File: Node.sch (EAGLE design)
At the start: 72 parts, among them J1 AVR_SPI_PRG_6NS, J2 M04X2, Q1 PMR280UN, Q2 PMR280UN, Q3 PMR280UN, SW1 KSS, U1 ATMEGA32U4, U2 BLUETOOTH-RN41", U4 L3GD20, U9 RCLAMP0502A, X1 USBSMD

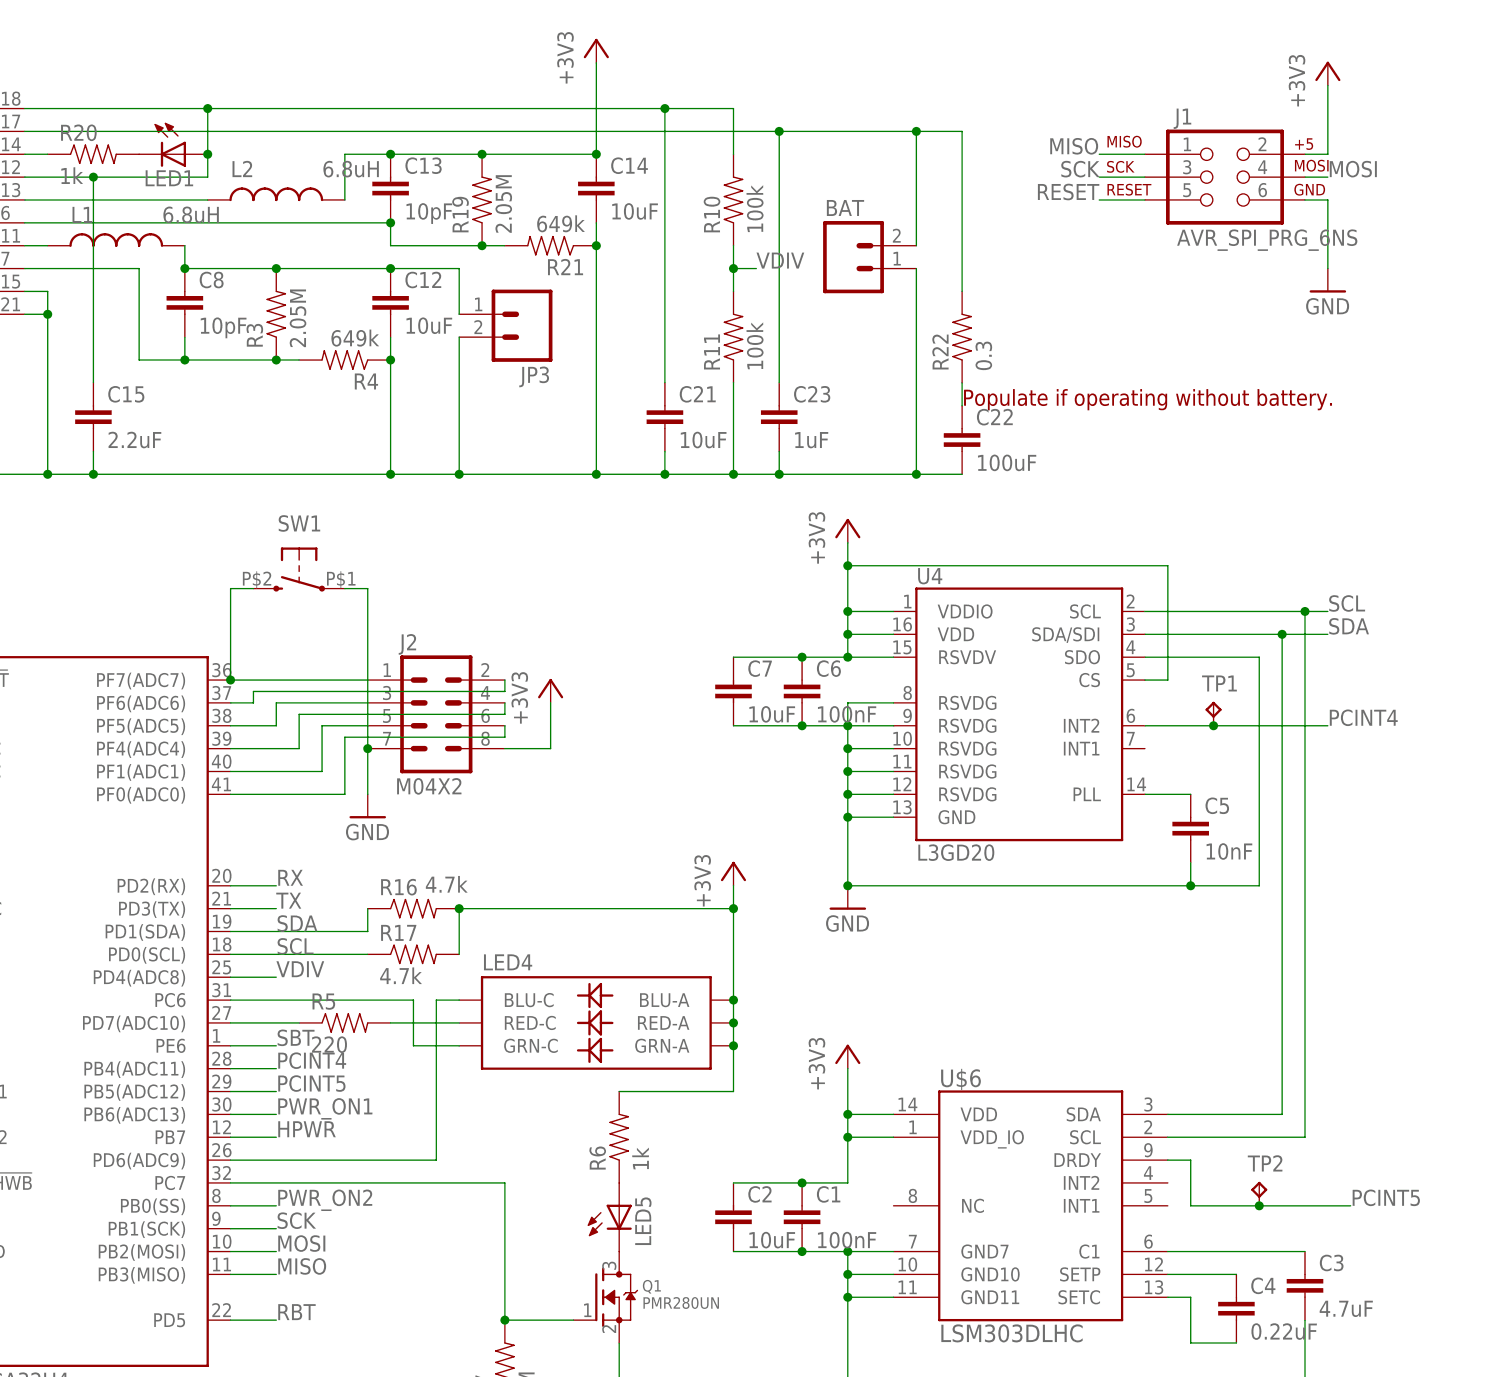
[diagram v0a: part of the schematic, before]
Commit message: it all sort of fits in the box
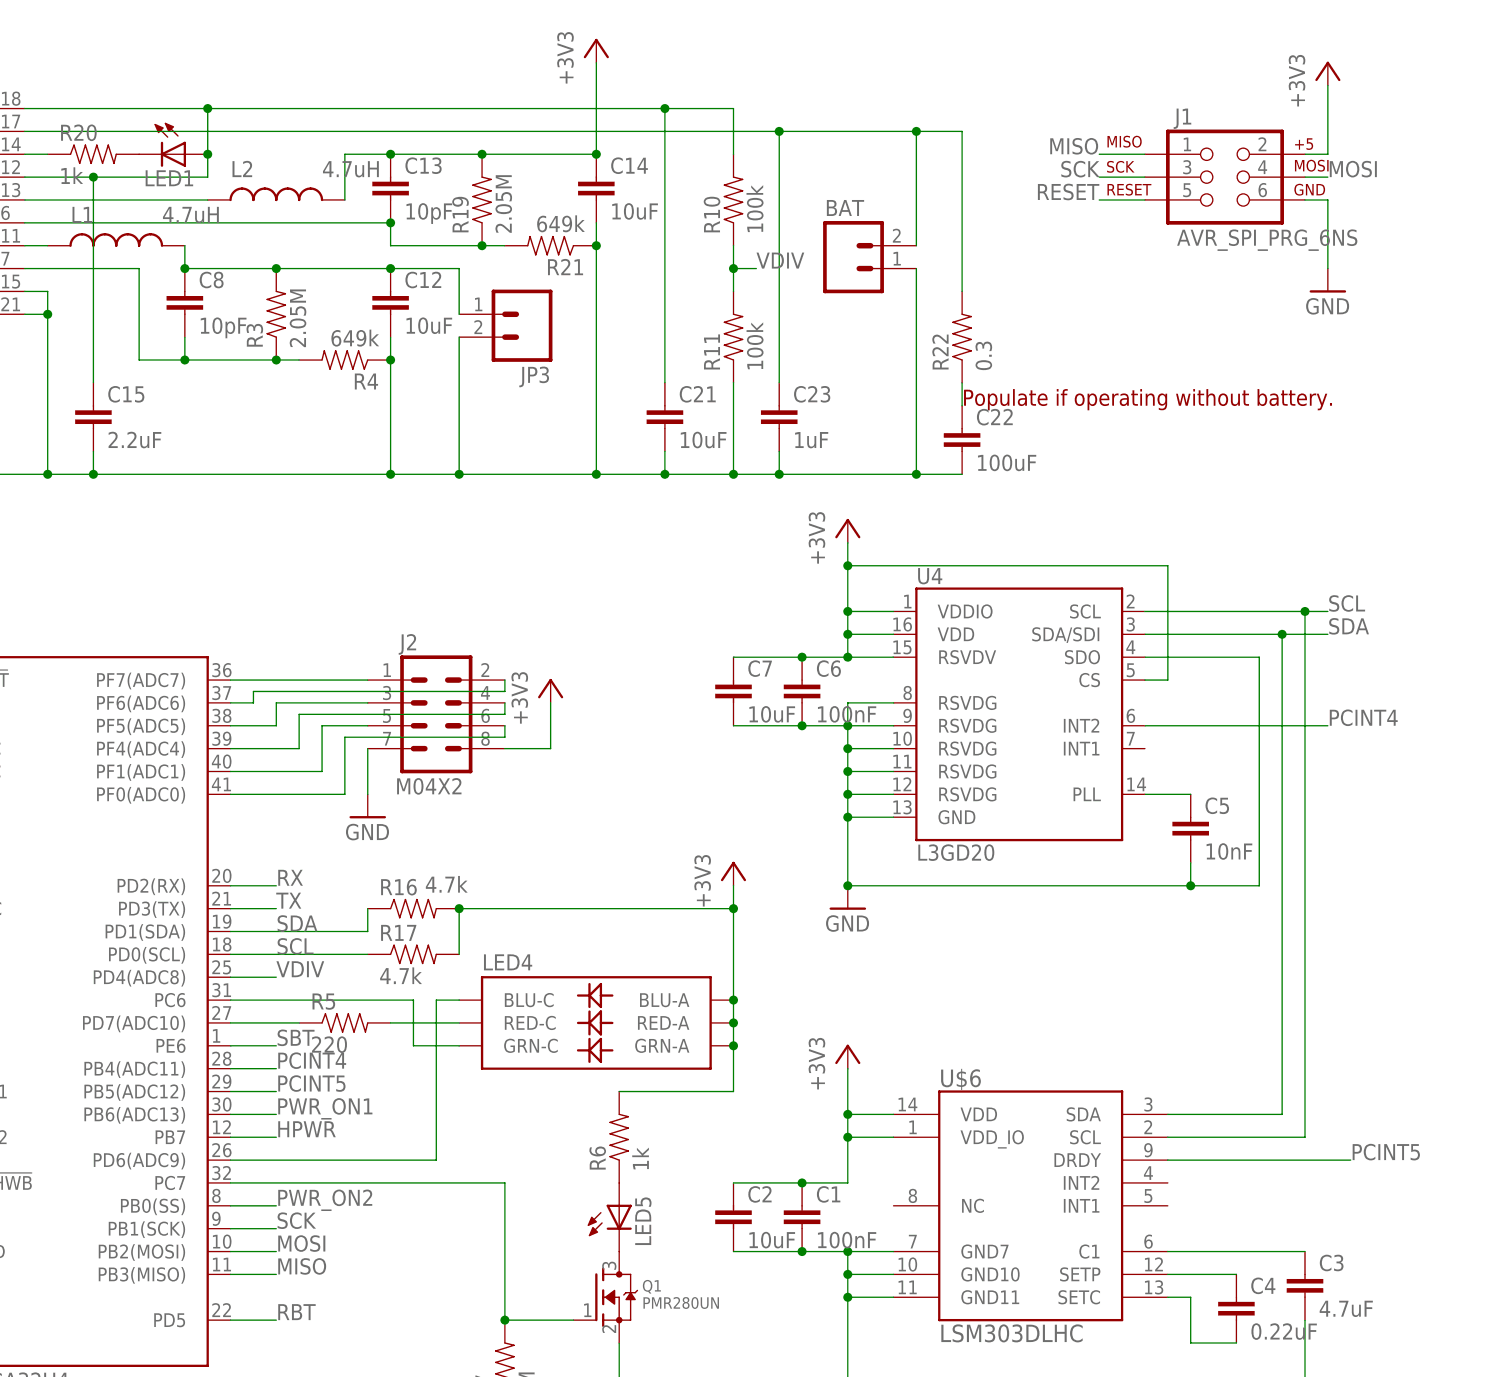
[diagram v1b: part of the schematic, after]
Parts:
- removed SW1: KSS, adjacent-reality:KSS
- removed TP1, TP2: TPTP06R, testpad:TPTP06R
- L1, L2: value 6.8uH -> 4.7uH; device adjacent-reality:INDUCTOR -> adjacent-reality:INDUCTORVLS2016
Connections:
- net GND: no longer SW1.1
- net N$28: no longer SW1.3
- net PCINT4: no longer TP1.TP
- net PCINT5: no longer TP2.TP
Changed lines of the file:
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@@
 <part name="R9" library="SparkFun" deviceset="RESISTOR" device="0402-RES" value="22"/>
 <part name="GND7" library="supply1" deviceset="GND" device=""/>
-<part name="SW1" library="adjacent-reality" deviceset="KSS" device=""/>
 <part name="HWB" library="adjacent-reality" deviceset="KSS" device=""/>
 <part name="C16" library="SparkFun" deviceset="CAP" device="0402-CAP" value="100nF"/>
@@
 <part name="R18" library="SparkFun" deviceset="RESISTOR" device="0402-RES" value="10k"/>
 <part name="U9" library="adjacent-reality" deviceset="RCLAMP0502A" device=""/>
-<part name="TP1" library="testpad" deviceset="TP" device="TP06R"/>
-<part name="TP2" library="testpad" deviceset="TP" device="TP06R"/>
 <part name="GND9" library="supply1" deviceset="GND" device=""/>
 <part name="LED1" library="SparkFun" deviceset="LED" device="0603"/>
@@
 <part name="C23" library="SparkFun" deviceset="CAP" device="0402-CAP" value="1uF"/>
 <part name="U$6" library="adjacent-reality" deviceset="LSM303DLHC" device=""/>
-<part name="L1" library="adjacent-reality" deviceset="INDUCTOR" device="" value="6.8uH"/>
-<part name="L2" library="adjacent-reality" deviceset="INDUCTOR" device="" value="6.8uH"/>
+<part name="L1" library="adjacent-reality" deviceset="INDUCTOR" device="VLS2016" value="4.7uH"/>
+<part name="L2" library="adjacent-reality" deviceset="INDUCTOR" device="VLS2016" value="4.7uH"/>
 <part name="JP1" library="SparkFun-Connectors" deviceset="M02" device="PTH"/>
 </parts>
@@
 <instance part="R9" gate="G$1" x="73.66" y="96.52"/>
 <instance part="GND7" gate="1" x="33.02" y="91.44"/>
-<instance part="SW1" gate="G$1" x="147.32" y="144.78" rot="MR0"/>
 <instance part="HWB" gate="G$1" x="48.26" y="134.62" smashed="yes" rot="MR0">
 <attribute name="NAME" x="50.8" y="140.97" size="1.778" layer="95" rot="MR0"/>
@@
 <instance part="R18" gate="G$1" x="55.88" y="139.7" rot="R90"/>
 <instance part="U9" gate="G$1" x="50.8" y="99.06"/>
-<instance part="TP1" gate="G$1" x="248.92" y="132.08"/>
-<instance part="TP2" gate="G$1" x="254" y="78.74"/>
 <instance part="GND9" gate="1" x="154.94" y="119.38"/>
 <instance part="LED1" gate="G$1" x="134.62" y="193.04" rot="R270"/>
@@
 <pinref part="J2" gate="G$1" pin="7"/>
 <wire x1="154.94" y1="121.92" x2="154.94" y2="127" width="0.1524" layer="91"/>
-<wire x1="154.94" y1="144.78" x2="154.94" y2="127" width="0.1524" layer="91"/>
-<junction x="154.94" y="127"/>
-<pinref part="SW1" gate="G$1" pin="1"/>
-<wire x1="154.94" y1="144.78" x2="152.4" y2="144.78" width="0.1524" layer="91"/>
 </segment>
 </net>
@@
 <segment>
 <pinref part="U4" gate="G$1" pin="INT2"/>
-<wire x1="241.3" y1="129.54" x2="248.92" y2="129.54" width="0.1524" layer="91"/>
 <label x="261.62" y="129.54" size="1.778" layer="95"/>
-<pinref part="TP1" gate="G$1" pin="TP"/>
-<wire x1="248.92" y1="129.54" x2="261.62" y2="129.54" width="0.1524" layer="91"/>
-<junction x="248.92" y="129.54"/>
+<wire x1="241.3" y1="129.54" x2="261.62" y2="129.54" width="0.1524" layer="91"/>
 </segment>
 </net>
@@
 </segment>
 <segment>
-<label x="264.16" y="76.2" size="1.778" layer="95"/>
-<pinref part="TP2" gate="G$1" pin="TP"/>
-<wire x1="254" y1="76.2" x2="264.16" y2="76.2" width="0.1524" layer="91"/>
-<wire x1="254" y1="76.2" x2="246.38" y2="76.2" width="0.1524" layer="91"/>
-<wire x1="246.38" y1="76.2" x2="246.38" y2="81.28" width="0.1524" layer="91"/>
-<junction x="254" y="76.2"/>
+<label x="264.16" y="81.28" size="1.778" layer="95"/>
+<wire x1="243.84" y1="81.28" x2="264.16" y2="81.28" width="0.1524" layer="91"/>
 <pinref part="U$6" gate="G$1" pin="DRDY"/>
-<wire x1="246.38" y1="81.28" x2="243.84" y2="81.28" width="0.1524" layer="91"/>
 </segment>
 </net>
@@
 <pinref part="J2" gate="G$1" pin="1"/>
 <wire x1="139.7" y1="134.62" x2="154.94" y2="134.62" width="0.1524" layer="91"/>
-<wire x1="139.7" y1="144.78" x2="139.7" y2="134.62" width="0.1524" layer="91"/>
-<junction x="139.7" y="134.62"/>
-<pinref part="SW1" gate="G$1" pin="3"/>
-<wire x1="139.7" y1="144.78" x2="142.24" y2="144.78" width="0.1524" layer="91"/>
-</segment>
-</net>
+</segment>
+</net>
